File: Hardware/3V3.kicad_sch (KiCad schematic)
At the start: 12 parts, among them U4 TPS63020DSJR

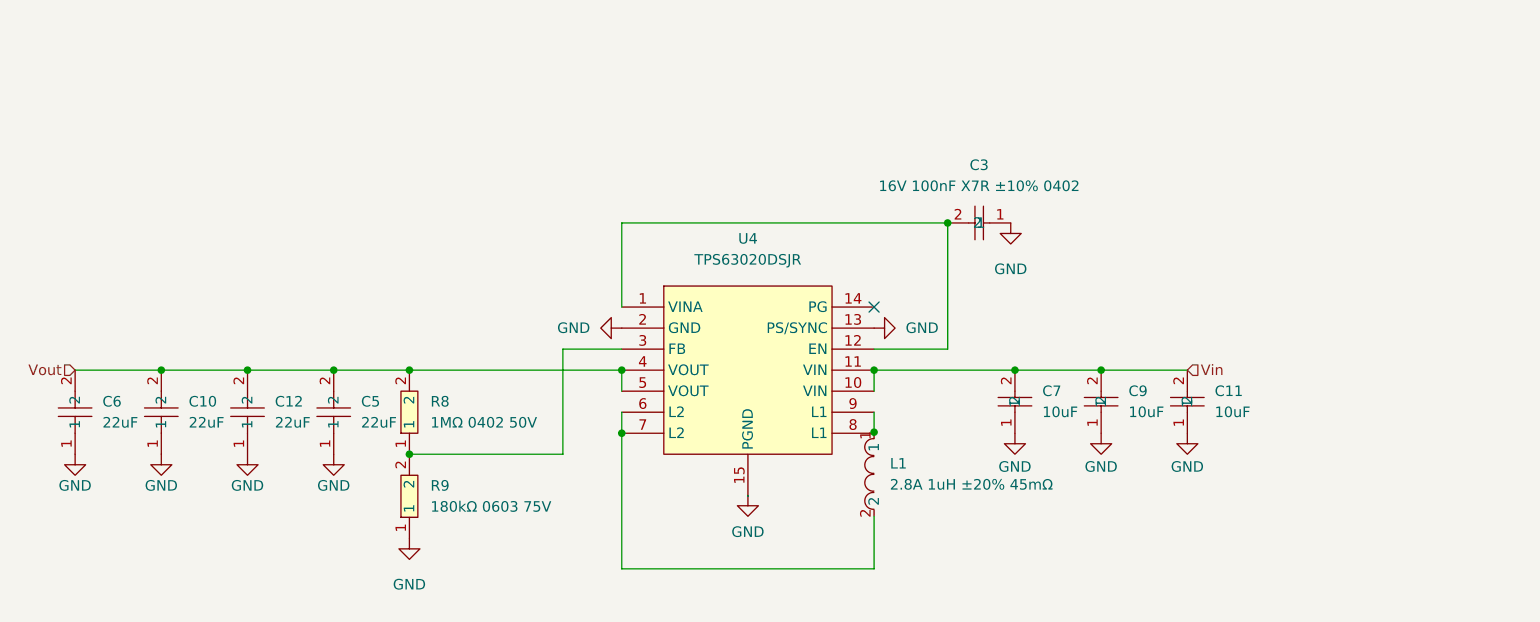
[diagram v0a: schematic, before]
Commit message: PCB V2
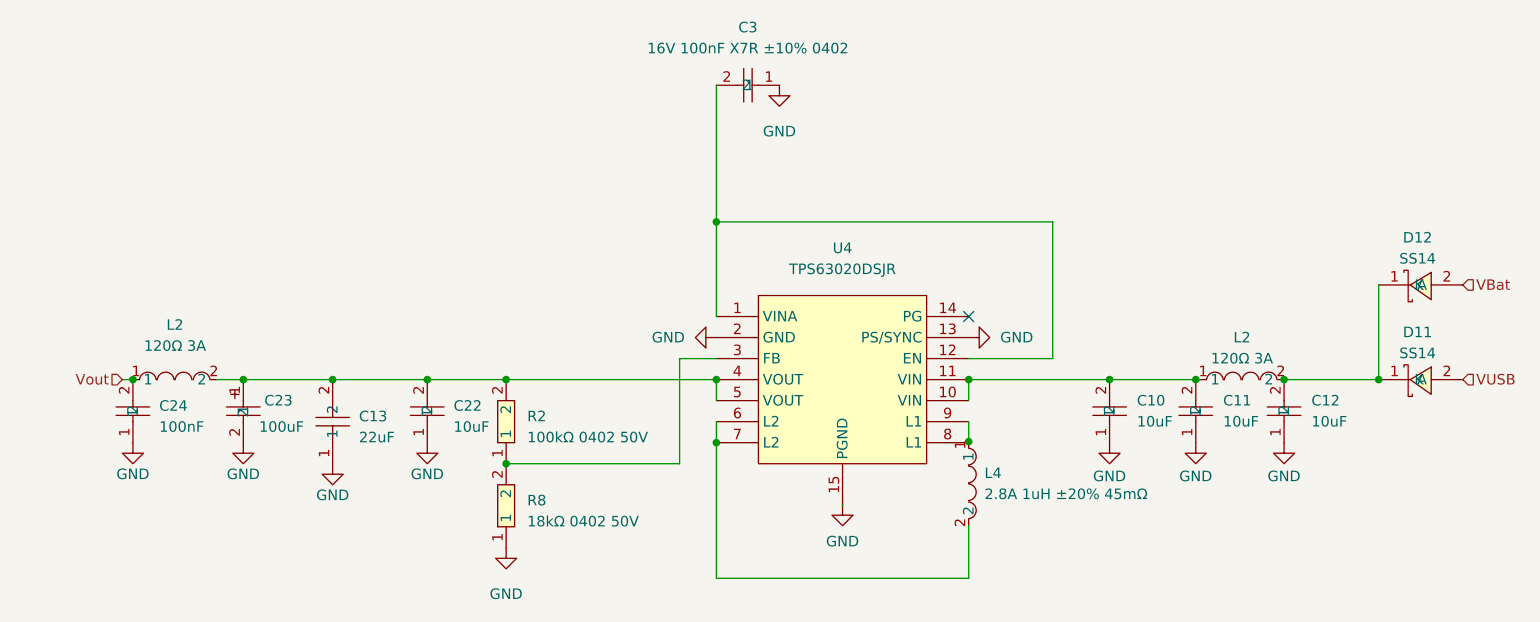
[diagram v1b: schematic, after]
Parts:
- removed C10, C12, C5, C6: 22uF, easyeda2kicad:C0603, symbol easyeda2kicad:6.3V 22uF X5R ±20% 0603
- removed R8: 1MΩ 0402 50V, easyeda2kicad:R0402, symbol easyeda2kicad:1MΩ 0402 50V
- removed R9: 180kΩ 0603 75V, easyeda2kicad:R0603, symbol easyeda2kicad:180kΩ 0603 75V
- added C13: 22uF, easyeda2kicad:C0603, symbol easyeda2kicad:6.3V 22uF X5R ±20% 0603
- added C22: 10uF, easyeda2kicad:C0402, symbol easyeda2kicad: 6.3V 10uF X5R ±20% 0402
- added C23: 100uF, easyeda2kicad:CAP-SMD_L3.5-W2.8, symbol easyeda2kicad:100uF 6.3V Tantal 3528
- added C24: 100nF, easyeda2kicad:C0402_NEW, symbol easyeda2kicad:16V 100nF X7R ±10% 0402
- added D11, D12: SS14, easyeda2kicad:SMA_L4.2-W2.6-LS5.3-RD, symbol easyeda2kicad:SS14
- added L2 (x2): 120Ω 3A, easyeda2kicad:L1206, symbol easyeda2kicad:120Ω 3A
- added R2: 100kΩ 0402 50V, easyeda2kicad:R0402, symbol easyeda2kicad:100kΩ 0402 50V
- added R8: 18kΩ 0402 50V, easyeda2kicad:R0402, symbol easyeda2kicad:18kΩ 0402 50V
- renumbered C7 to C10, C9 to C11, C11 to C12, L1 to L4
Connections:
- net GND: now also C13.1, C22.1, C23.2, C24.1, R8.1
- net Vout: now also C24.2, L2.1; no longer U4.4 (VOUT), U4.5 (VOUT)
- net at U4.3 (FB): now also R2.1, R8.2
- net Vin: no longer names the net of C10.2, C11.2, U4.10 (VIN), U4.11 (VIN)
- net Vin: now also L2.1; no longer C12.2
- new net: C12.2, D11.1 (K), D12.1 (K), L2.2
- new net: C13.2, C22.2, C23.1, L2.2, R2.2, U4.4 (VOUT), U4.5 (VOUT)
- new net VBat: D12.2 (A)
- new net VUSB: D11.2 (A)
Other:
- moved on the sheet: C10, C11, C12, C3, L4, U4
